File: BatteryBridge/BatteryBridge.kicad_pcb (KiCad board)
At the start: 2 copper layers, 26.4 x 52.2 mm, 24 parts, among them IC1 MAX1595EUA50+, J1 JST_PH, J2 USB_A, J3 Conn_02x20_Odd_Even, Q1 Q_PMOS_GSD, U1 MCP73832-2-OT, U2 LTC4412xS6

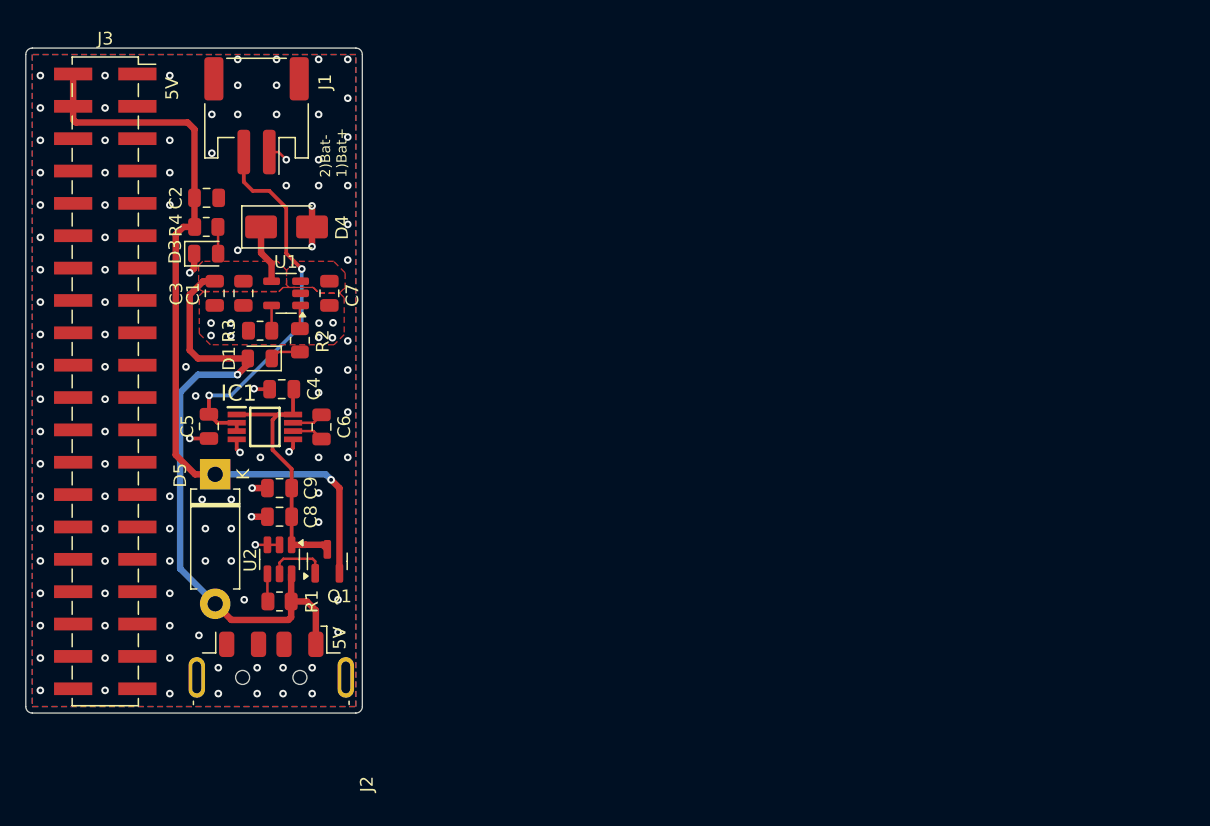
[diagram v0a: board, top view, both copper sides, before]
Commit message: Finished V1.1, added gerbers/drills
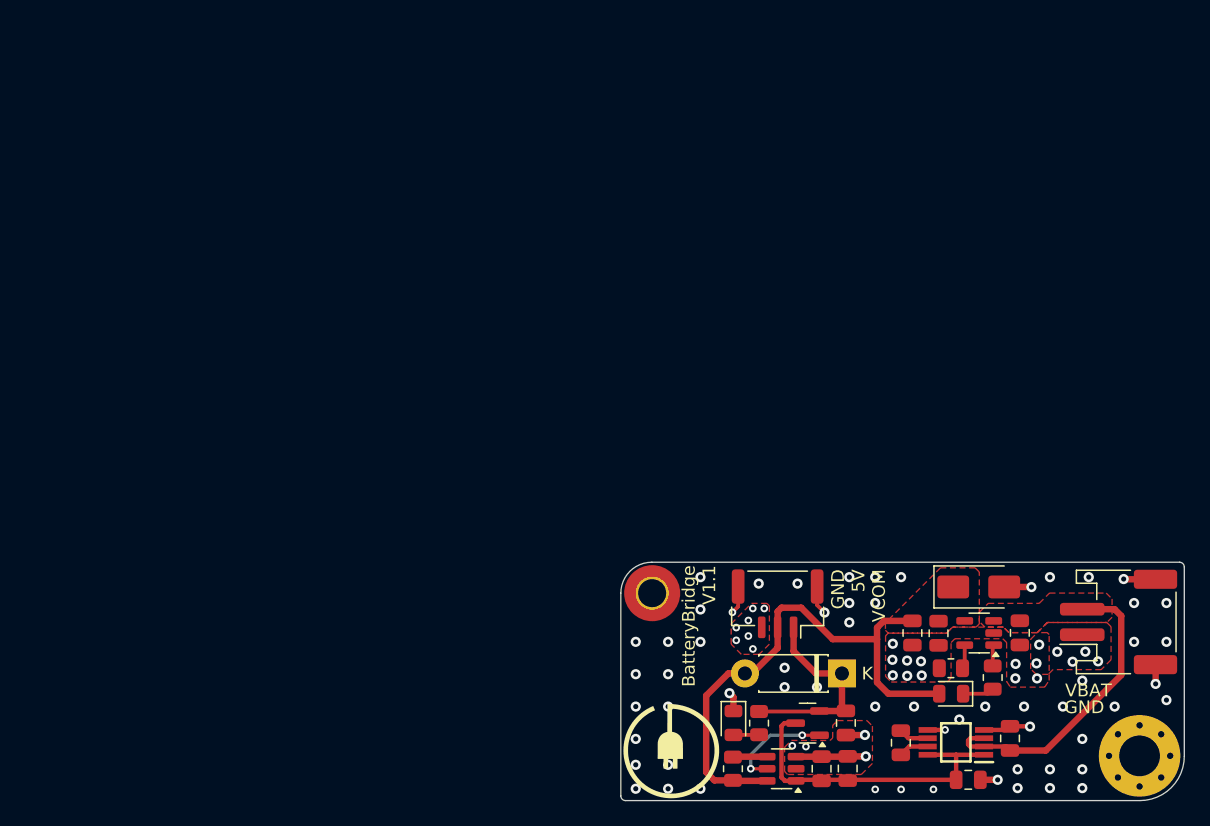
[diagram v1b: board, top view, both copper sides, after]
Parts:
- removed J2: USB_A, Connector_USB:USB_A_Molex_48037-2200_Horizontal
- removed J3: Conn_02x20_Odd_Even, Connector_PinSocket_2.54mm:PinSocket_2x20_P2.54mm_Vertical_SMD
- added G***: LOGO, Logo:GLogoSmall, F.Cu at (111.5, 92.4)
- added H1: MH, MountingHole:MountingHole_3.2mm_M3_Pad_Via, F.Cu at (148.3, 92.8)
- added H2: MH, MountingHole:MountingHole_2.2mm_M2_Pad_TopOnly, F.Cu at (110.0, 80.0)
- added J4: JST_BH, Connector_JST:JST_GH_SM03B-GHS-TB_1x03-1MP_P1.25mm_Horizontal, F.Cu at (119.8, 80.8)
- C1, C7, C9: value 4.7uF -> 4.7uF 0805 X5R 25V (or better)
- C2: value 10uF -> 10uF 16V X5R (or better)
- C3, C8: value 100n -> 100nF (0.1uF) 0805 X5R 10V (or better)
- C4, C5: value 2u2 -> 2.2uF 0805 X5R 25V (or better)
- C6: value 0u47 -> 0.47uF 0805 X7R 50V (or better)
- D1, D3: value GREEN -> LED GREEN CLEAR 0805 SMD
- D5: footprint Diode_THT:D_DO-15_P10.16mm_Horizontal -> Diode_THT:D_DO-41_SOD81_P7.62mm_Horizontal
- R1: value 470k -> 470k 0805 1%
- R2, R4: value 470 -> 470R 0805 1%
- R3: value 2k -> 2k 0805 1%
- moved J1 78.5 mm to (146.6, 82.3), turned to 90 degrees
- moved C5 67.5 mm to (138.1, 91.4), turned to 90 degrees
- moved C2 64.9 mm to (125.2, 90.2), turned to -90 degrees
- moved C3 62.8 mm to (132.5, 83.1)
- moved C4 62.0 mm to (134.8, 94.7), turned to 0 degrees
- moved D4 61.2 mm to (135.6, 79.5)
- moved U1 60.6 mm to (135.7, 83.1)
- moved R2 60.5 mm to (136.7, 86.6)
- moved C7 60.4 mm to (138.9, 83.1)
- moved R3 60.4 mm to (133.4, 85.9)
- moved D1 60.3 mm to (133.5, 87.9)
- moved IC1 59.6 mm to (133.8, 91.7), turned to 180 degrees
- moved C1 58.9 mm to (130.4, 83.1)
- moved R4 58.3 mm to (118.4, 90.2), turned to -90 degrees
- moved D3 55.4 mm to (116.4, 90.2), turned to -90 degrees
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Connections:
- net /VIN_RASP renamed VCOM
- net Net-(D1-K) renamed /R_LED_BAT
- net Net-(D3-A) renamed /R_LED
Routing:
- net VCOM: track 60.7 -> 16.7 mm, vias 1 -> 0
- net +5V: track 55.5 -> 42.6 mm, vias 1 -> 0
- net GND: track 15.8 -> 25.6 mm, vias 120 -> 88
- net /VBat: track 30.4 -> 24.2 mm, vias 2 -> 0
- net /BUCK_OUT: track 21.6 -> 25.5 mm
- net /GATE: track 4.83 -> 8.41 mm, vias 0 -> 2
- net /STAT_LTC: track 2.19 -> 2.70 mm
- added copper zone on In1.Cu, net GND
- added copper zone on In2.Cu, net GND
- removed copper zone on B.Cu, net GND
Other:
- board size 26.4 x 52.2 mm -> 44.2 x 18.7 mm
- copper layers 2 -> 4
- board text added: "BatteryBridge V1.1"
- board text added: "GND"
- board text added: "GND 5V VCOM"
- board text added: "VBAT"
- board text removed: "2)Bat- 1)Bat+"
- board text removed: "5V"
